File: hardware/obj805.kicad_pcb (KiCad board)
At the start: 2 copper layers, 65 x 56.5 mm, 41 parts, among them J0 Conn_with_rapi, U1 l293d

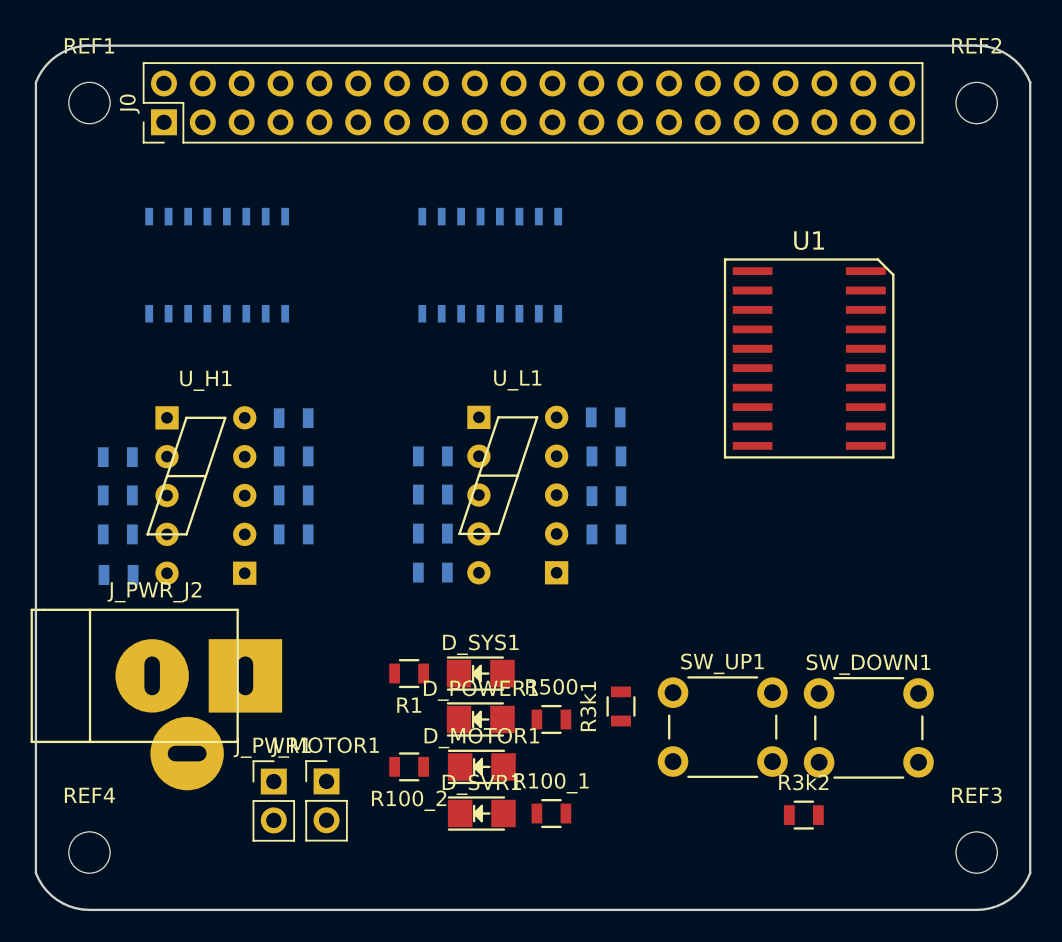
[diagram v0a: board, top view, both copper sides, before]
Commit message: update
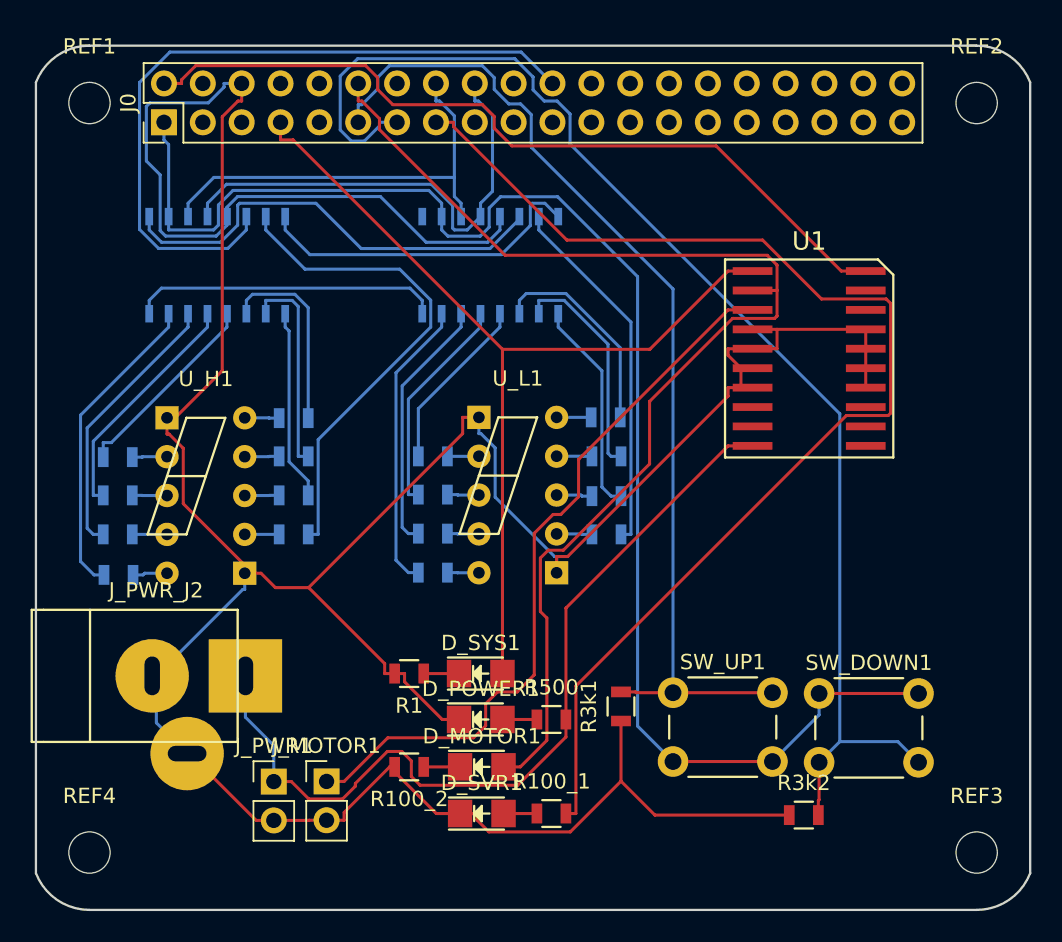
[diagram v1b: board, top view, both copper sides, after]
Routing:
- net Net-(D_POWER1-Pad1): track 0.00 -> 231.6 mm
- net Net-(J0-Pad1): track 0.00 -> 97.3 mm
- net Net-(J0-Pad13): track 0.00 -> 85.1 mm
- net Net-(J0-Pad15): track 0.00 -> 78.9 mm
- net Net-(D_MOTOR1-Pad2): track 0.00 -> 78.4 mm
- net Net-(J0-Pad11): track 0.00 -> 67.3 mm
- net Net-(D_SYS1-Pad2): track 0.00 -> 61.0 mm
- net Net-(J_PWR1-Pad1): track 0.00 -> 56.5 mm
- net Net-(J0-Pad2): track 0.00 -> 53.0 mm
- net Net-(J_MOTOR1-Pad1): track 0.00 -> 48.3 mm
- net Net-(J0-Pad22): track 0.00 -> 47.1 mm
- net Net-(R2-Pad2): track 0.00 -> 32.6 mm
- net Net-(J0-Pad18): track 0.00 -> 31.3 mm
- net Net-(UM_H1-Pad9): track 0.00 -> 29.4 mm
- net Net-(J0-Pad16): track 0.00 -> 28.5 mm
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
